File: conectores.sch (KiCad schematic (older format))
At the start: 31 parts, among them IC1 Corriente C, J5 TENSION

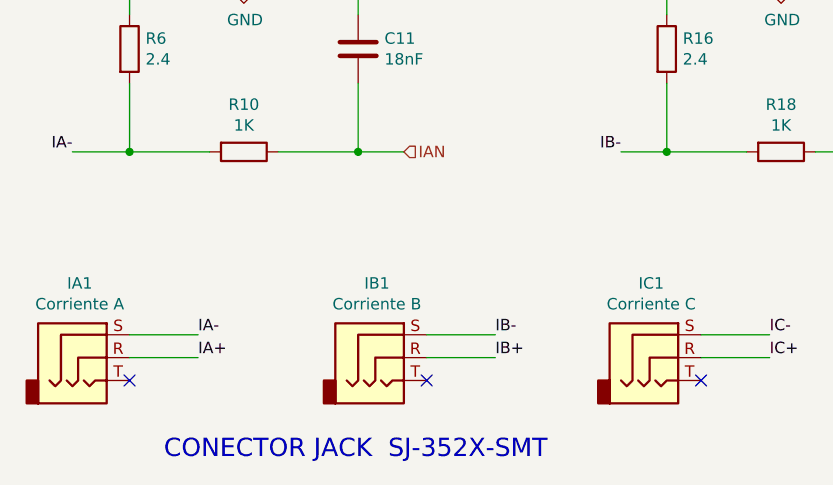
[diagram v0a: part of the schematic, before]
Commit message: Add files via upload
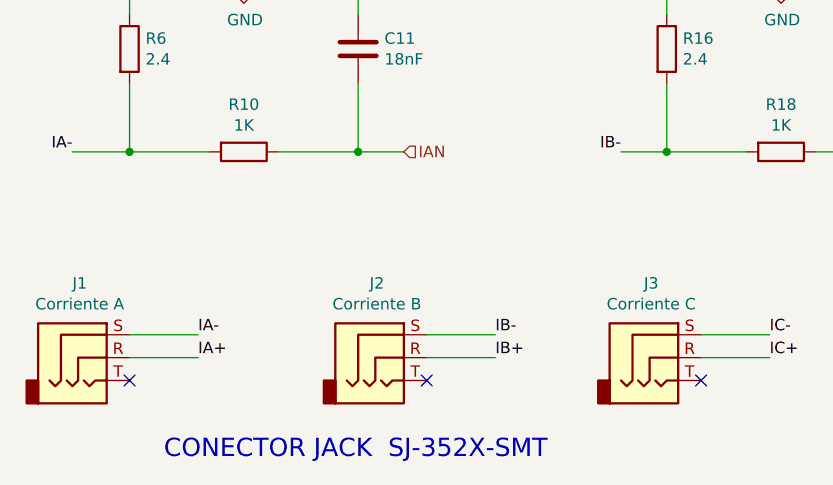
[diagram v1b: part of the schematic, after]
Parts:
- renumbered IA1 to J1, IB1 to J2, IC1 to J3
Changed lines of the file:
@@
 Configuración de Tensión
 $Comp
-L Connector:AudioJack3 IA1
+L Connector:AudioJack3 J1
 U 1 1 5EDFB80D
 P 2250 7000
-F 0 "IA1" H 2232 7325 50  0000 C CNN
+F 0 "J1" H 2232 7325 50  0000 C CNN
 F 1 "Corriente A" H 2232 7234 50  0000 C CNN
 F 2 "Connector_Audio:Jack_3.5mm_CUI_SJ-3523-SMT_Horizontal" H 2250 7000 50  0001 C CNN
@@
 $EndComp
 $Comp
-L Connector:AudioJack3 IB1
+L Connector:AudioJack3 J2
 U 1 1 5EDFC470
 P 3550 7000
-F 0 "IB1" H 3532 7325 50  0000 C CNN
+F 0 "J2" H 3532 7325 50  0000 C CNN
 F 1 "Corriente B" H 3532 7234 50  0000 C CNN
 F 2 "Connector_Audio:Jack_3.5mm_CUI_SJ-3523-SMT_Horizontal" H 3550 7000 50  0001 C CNN
@@
 $EndComp
 $Comp
-L Connector:AudioJack3 IC1
+L Connector:AudioJack3 J3
 U 1 1 5EDFCA1A
 P 4750 7000
-F 0 "IC1" H 4732 7325 50  0000 C CNN
+F 0 "J3" H 4732 7325 50  0000 C CNN
 F 1 "Corriente C" H 4732 7234 50  0000 C CNN
 F 2 "Connector_Audio:Jack_3.5mm_CUI_SJ-3523-SMT_Horizontal" H 4750 7000 50  0001 C CNN
